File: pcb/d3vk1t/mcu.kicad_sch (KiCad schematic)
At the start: 24 parts, among them IC1 STM32F412RETx, J1 Conn_01x03, J2 Conn_01x06, SW1 SW_Push, Y1 32.7680KHZ, Y2 24MHz

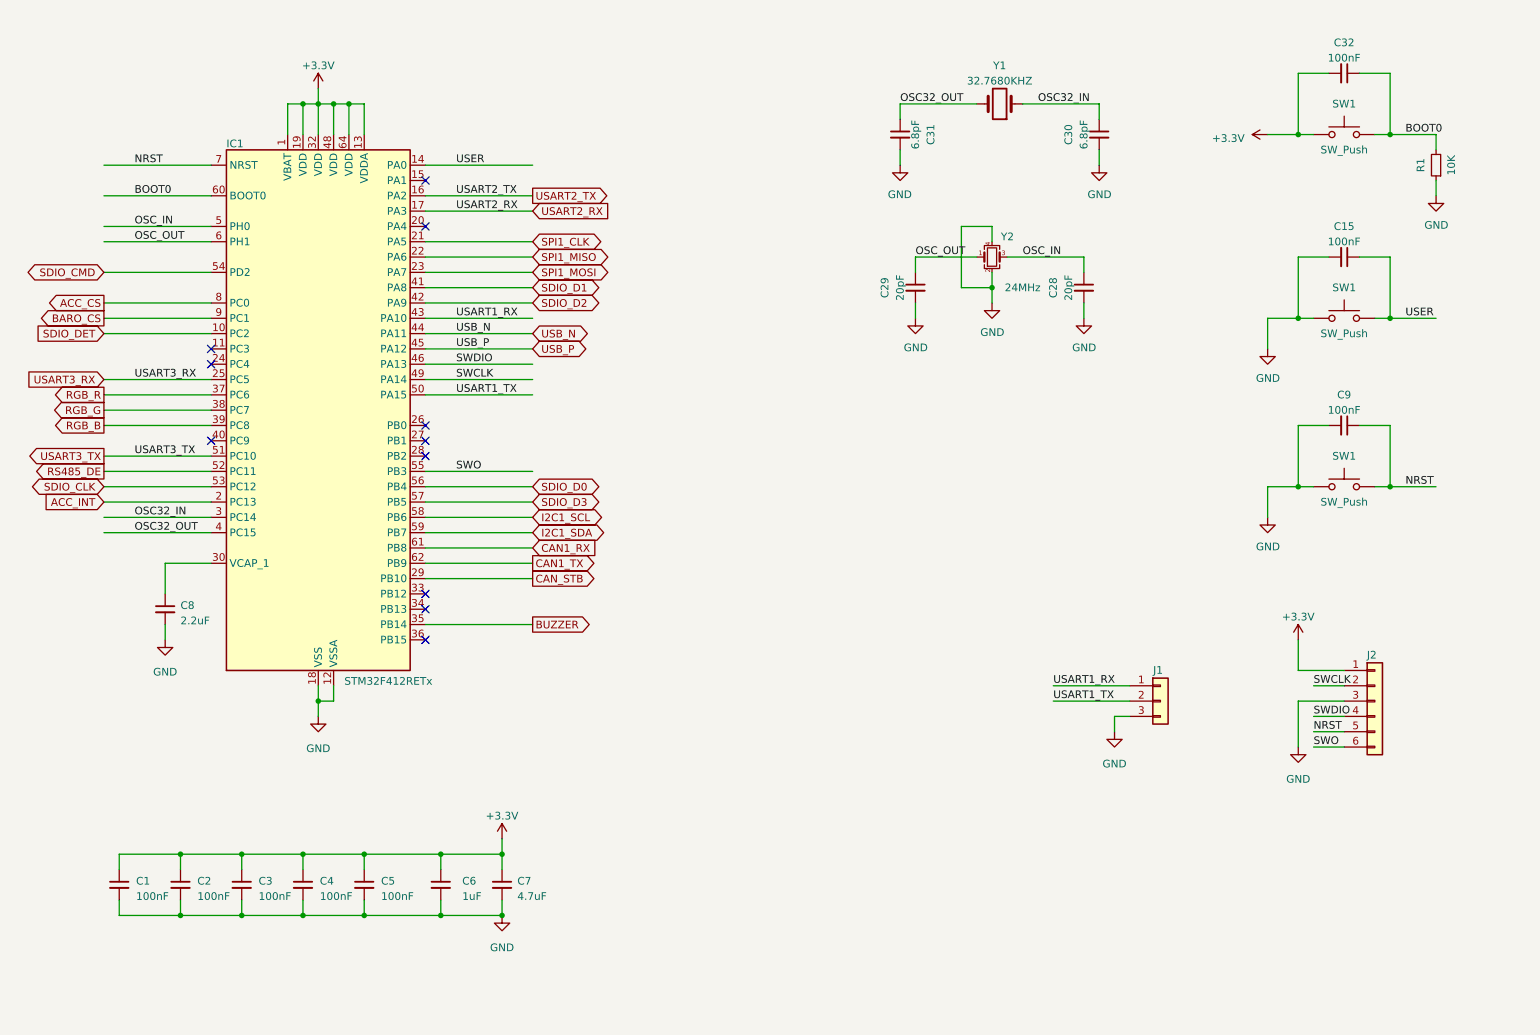
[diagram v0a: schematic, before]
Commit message: project update  - update pcb layout.  - update schmatics sheets.  - added manufacturing files.  - added documentation files.
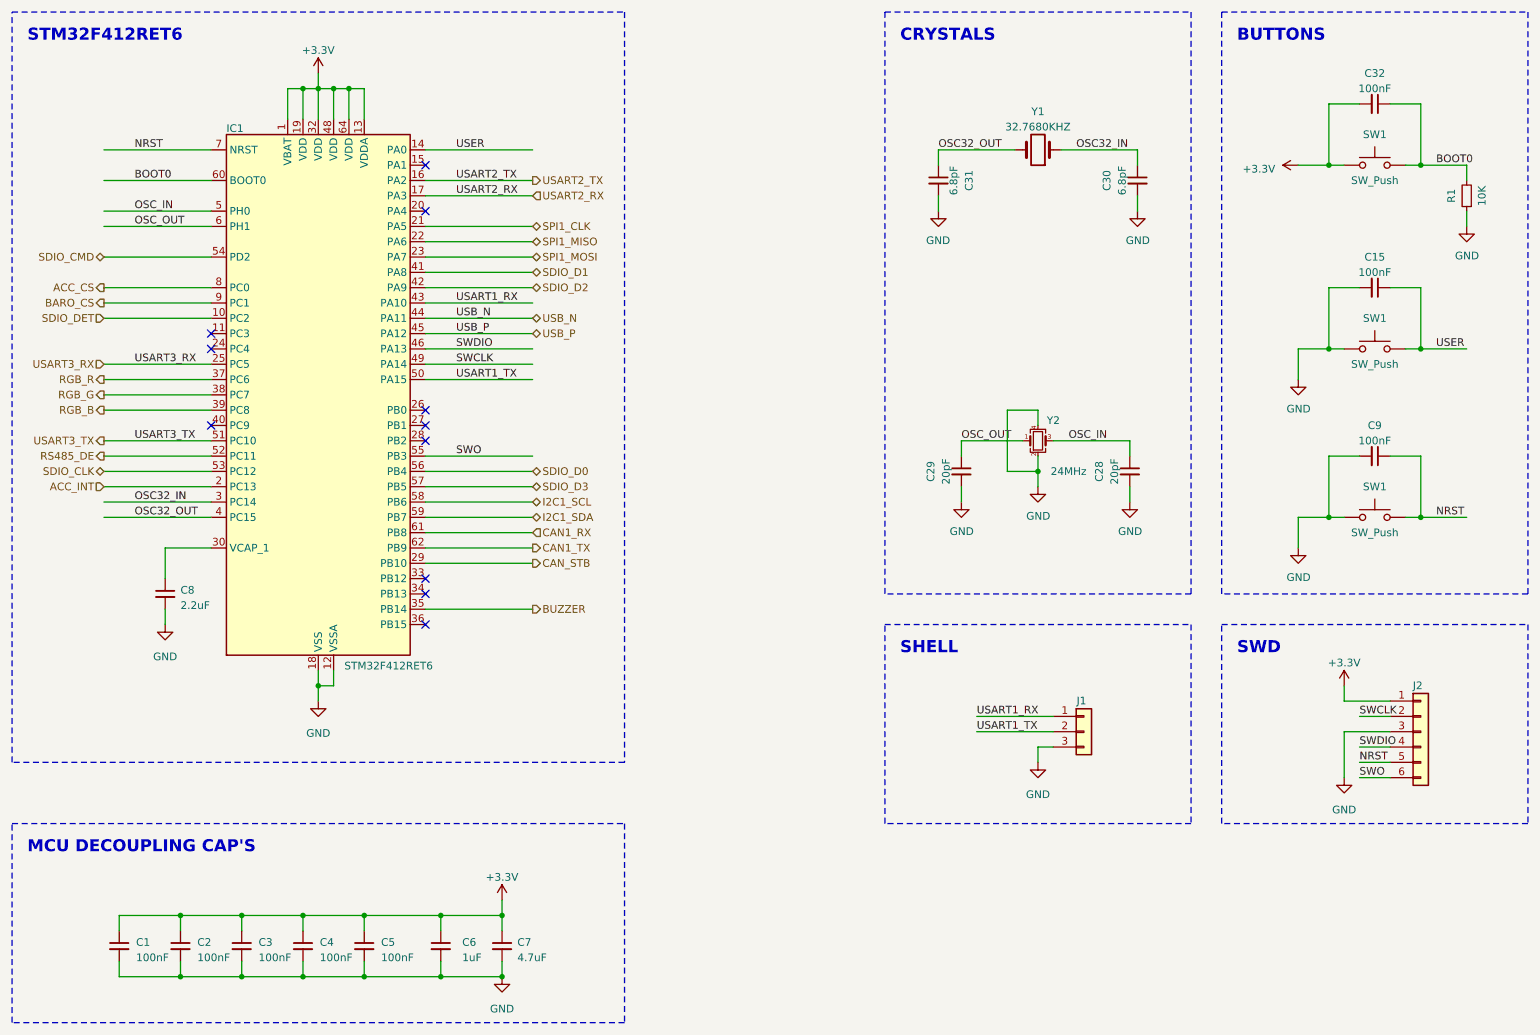
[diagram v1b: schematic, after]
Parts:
- IC1: value STM32F412RETx -> STM32F412RET6
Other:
- note added: "BUTTONS"
- note added: "CRYSTALS"
- note added: "MCU DECOUPLING CAP'S"
- note added: "SHELL"
- note added: "STM32F412RET6"
- note added: "SWD"
- title: (none) -> Microcontroller
- moved on the sheet: C1, C15, C2, C28, C29, C3, C30, C31, C32, C4, C5, C6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
